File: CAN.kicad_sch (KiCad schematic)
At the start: 8 parts, among them J2 Conn_01x02, U10 TCAN1044D, U8 MCP2518FDT-E/QBB, U9 TCAN1044D, Y1 40MHz

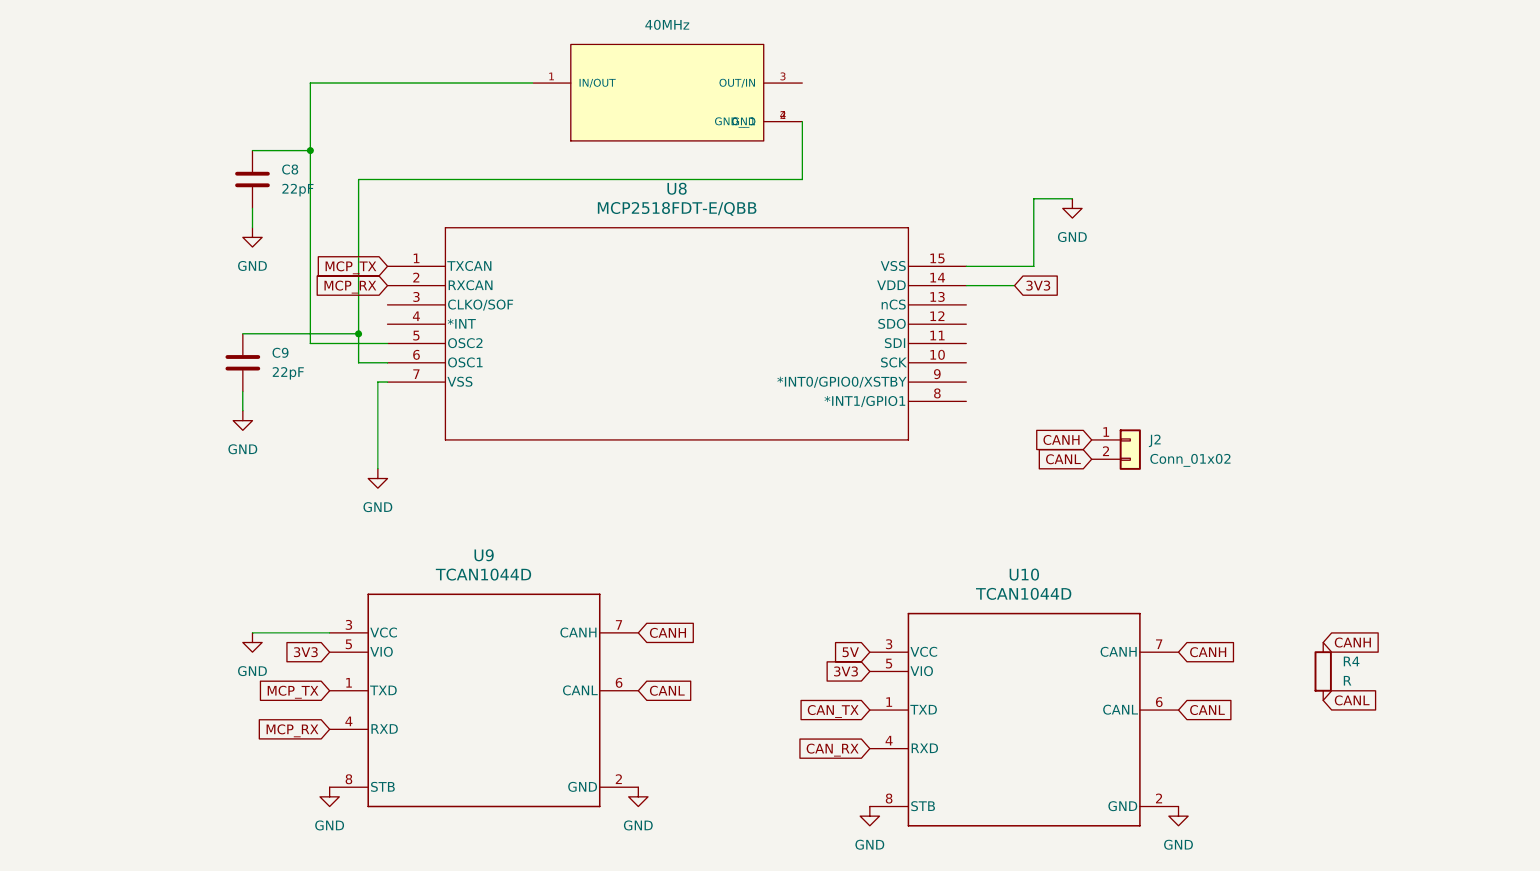
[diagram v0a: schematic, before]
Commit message: fixed stuff
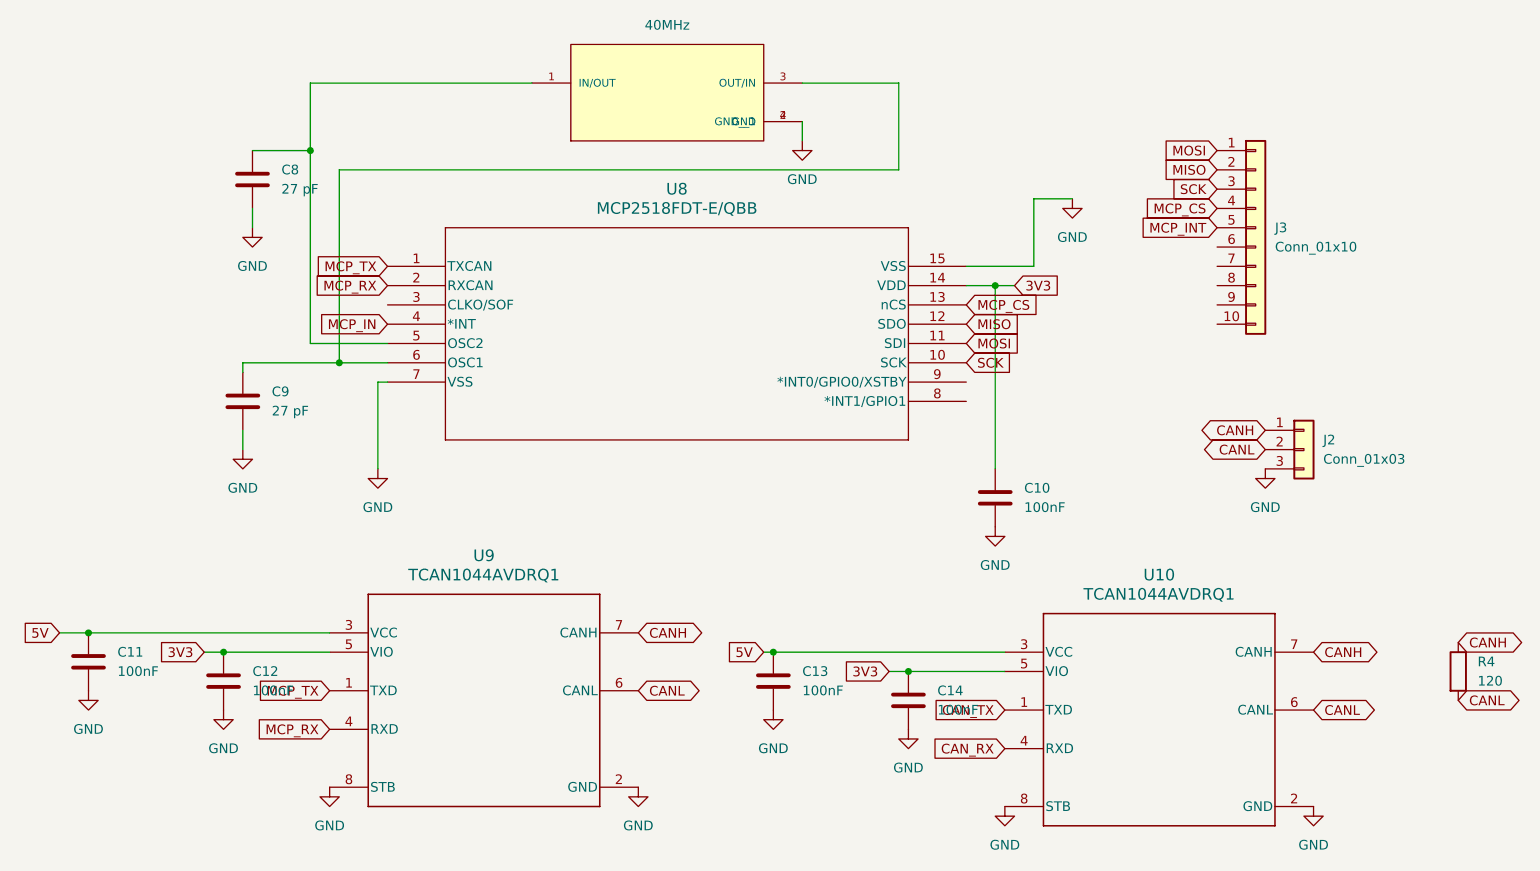
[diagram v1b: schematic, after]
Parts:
- removed J2: Conn_01x02, Package_DFN_QFN:QFN-56-1EP_8x8mm_P0.5mm_EP5.6x5.6mm_ThermalVias, symbol Connector_Generic:Conn_01x02
- added C10, C11, C12, C13, C14: 100nF, symbol Device:C
- added J2: Conn_01x03, TerminalBlock:TerminalBlock_MaiXu_MX126-5.0-03P_1x03_P5.00mm, symbol Connector_Generic:Conn_01x03
- added J3: Conn_01x10, Package_DFN_QFN:DFN-8-1EP_3x2mm_P0.5mm_EP1.7x1.4mm, symbol Connector_Generic:Conn_01x10
- C8, C9: value 22pF -> 27 pF; footprint (none) -> 0402
- R4: value R -> 120; footprint rov_sensors:Bosch_LGA-14_3x2.5mm_P0.5mm -> (none)
- U10, U9: value TCAN1044D -> TCAN1044AVDRQ1
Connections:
- net 3V3: now also C10.1, C12.1, C14.1
- net 5V: now also U9.3 (VCC), C11.1, C13.1
- net CANH: now also J2.1 (Pin_1)
- net CANL: now also J2.2 (Pin_2)
- net GND: now also Y1.2 (GND), Y1.4 (GND__1), C10.2, C11.2, C12.2, C13.2, C14.2, J2.3 (Pin_3); no longer U9.3 (VCC)
- net at C9.1, U8.6 (OSC1): now also Y1.3 (OUT/IN); no longer Y1.2 (GND), Y1.4 (GND__1)
- net SCK: now reaches U8.10 (SCK)
- net SCK: now also J3.3 (Pin_3)
- net MOSI: now reaches U8.11 (SDI)
- net MOSI: now also J3.1 (Pin_1)
- net MISO: now reaches U8.12 (SDO)
- net MISO: now also J3.2 (Pin_2)
- net MCP_CS: now reaches U8.13 (nCS)
- net MCP_CS: now also J3.4 (Pin_4)
- net MCP_IN: now reaches U8.4 (*INT)
- new net MCP_INT: J3.5 (Pin_5)
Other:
- moved on the sheet: C9, U10
